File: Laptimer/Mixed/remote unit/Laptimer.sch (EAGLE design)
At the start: 24 parts, among them IC4 74HC04D, IC5 NE555D, X2 GLX-S-88M

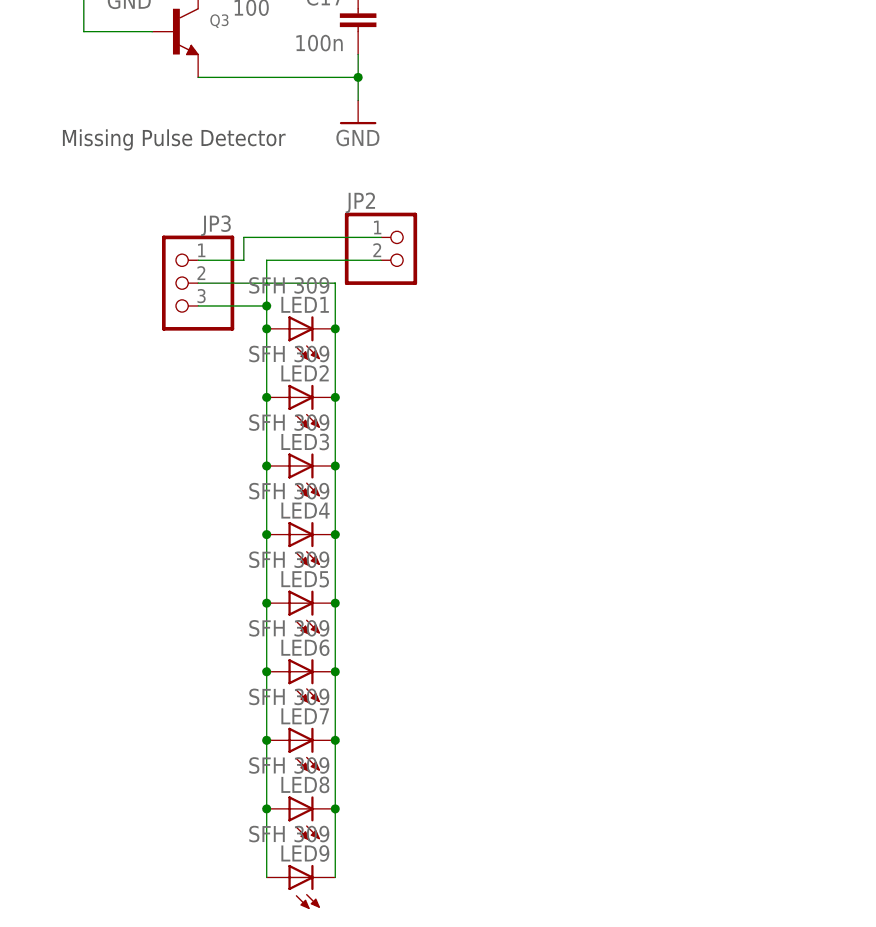
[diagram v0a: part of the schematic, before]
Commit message: more final board prepping for production
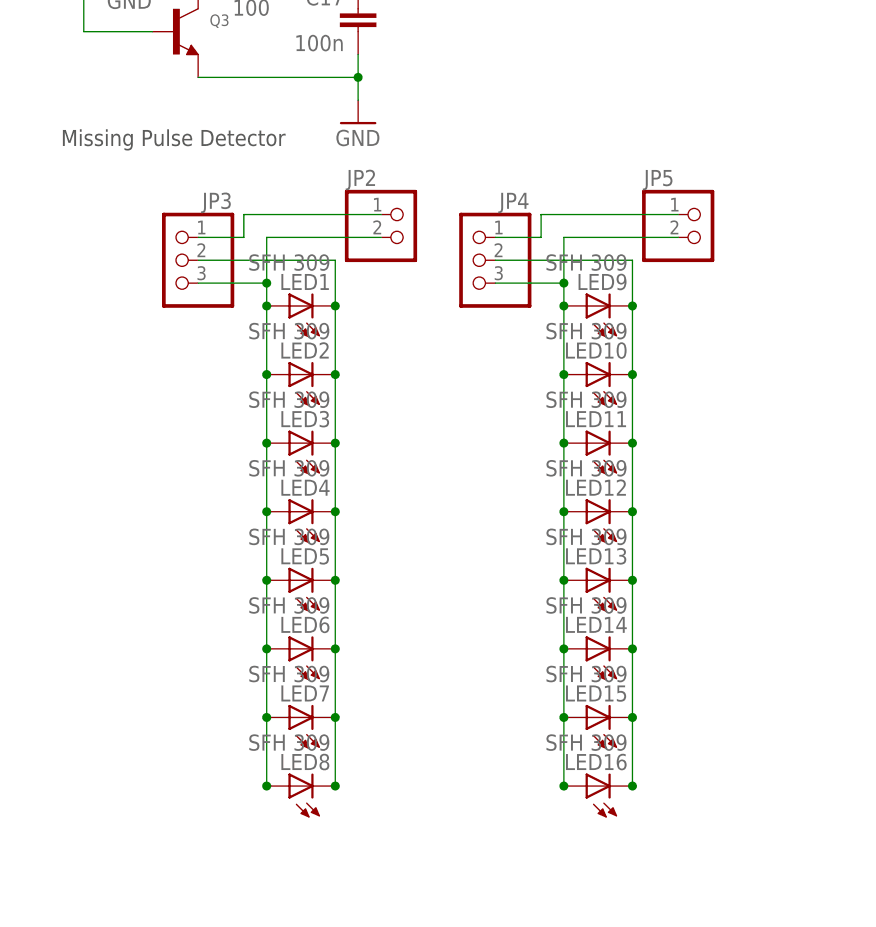
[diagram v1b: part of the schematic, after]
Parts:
- added JP4: (no value), adafruit:PINHD-1X3
- added JP5: (no value), microbuilder:HEADER-1X2ROUND
- added LED10, LED11, LED12, LED13, LED14, LED15, LED16: SFH 309, adafruit:LED3MM
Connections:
- new net INT1: JP4.2, LED10.C, LED11.C, LED12.C, LED13.C, LED14.C, LED15.C, LED16.C, LED9.C
- new net N$7: JP4.1, JP5.1
- new net N$8: JP4.3, JP5.2, LED10.A, LED11.A, LED12.A, LED13.A, LED14.A, LED15.A, LED16.A, LED9.A
- net INT: no longer LED9.C
- net N$40: no longer LED9.A
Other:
- moved on the sheet: JP2, JP3, LED1, LED2, LED3, LED4, LED5, LED6, LED7, LED8, LED9
